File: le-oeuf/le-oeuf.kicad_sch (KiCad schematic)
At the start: 76 parts, among them J1 S2B-PH-K-S, SW1 PG1425, SW10 PG1425, SW11 PG1425, SW12 PG1425, SW13 PG1425, SW14 PG1425, SW15 PG1425, SW16 PG1425, SW17 PG1425, SW18 PG1425, SW19 PG1425, SW2 PG1425, SW20 PG1425, SW21 PG1425, SW22 PG1425, SW23 PG1425, SW24 PG1425, SW25 PG1425, SW26 PG1425, SW27 PG1425, SW28 PG1425, SW29 PG1425, SW3 PG1425, SW30 PG1425, SW31 PG1425, SW32 PG1425, SW33 PG1425, SW34 PG1425, SW35 PG1425, SW36 PG1425, SW37 PCM12SMTR, SW4 PG1425, SW5 PG1425, SW6 PG1425, SW7 PG1425, SW8 PG1425, SW9 PG1425, U1 Seeeduino Xiao nRF52840, U2 74HC595D,118

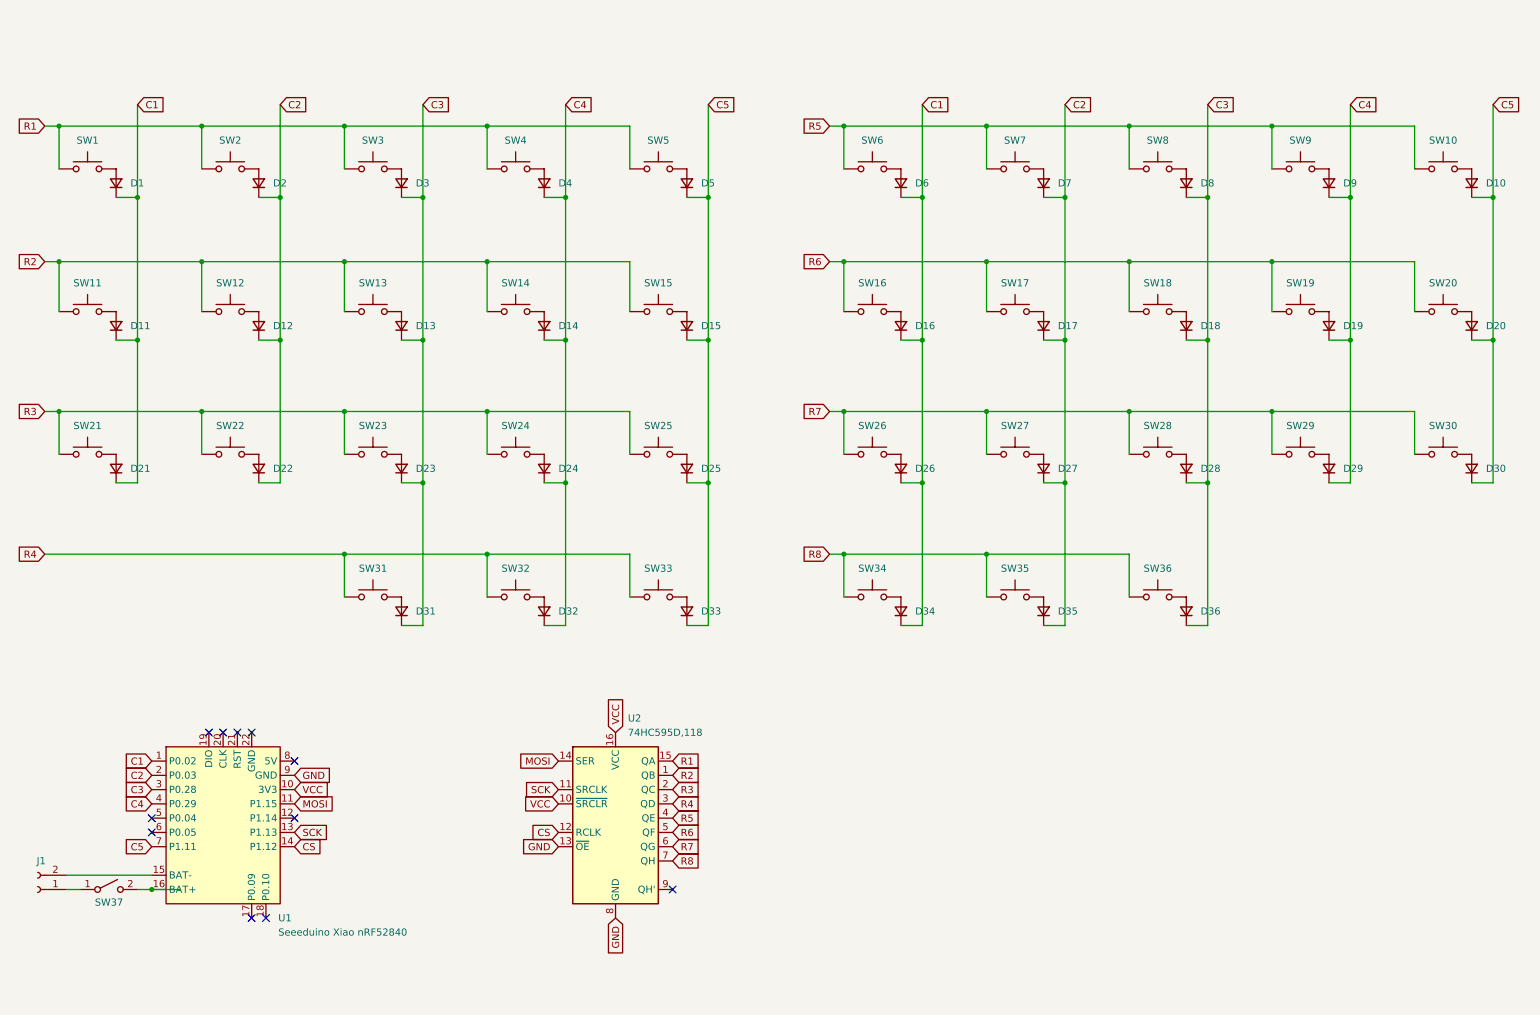
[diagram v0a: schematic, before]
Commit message: do not push this commit
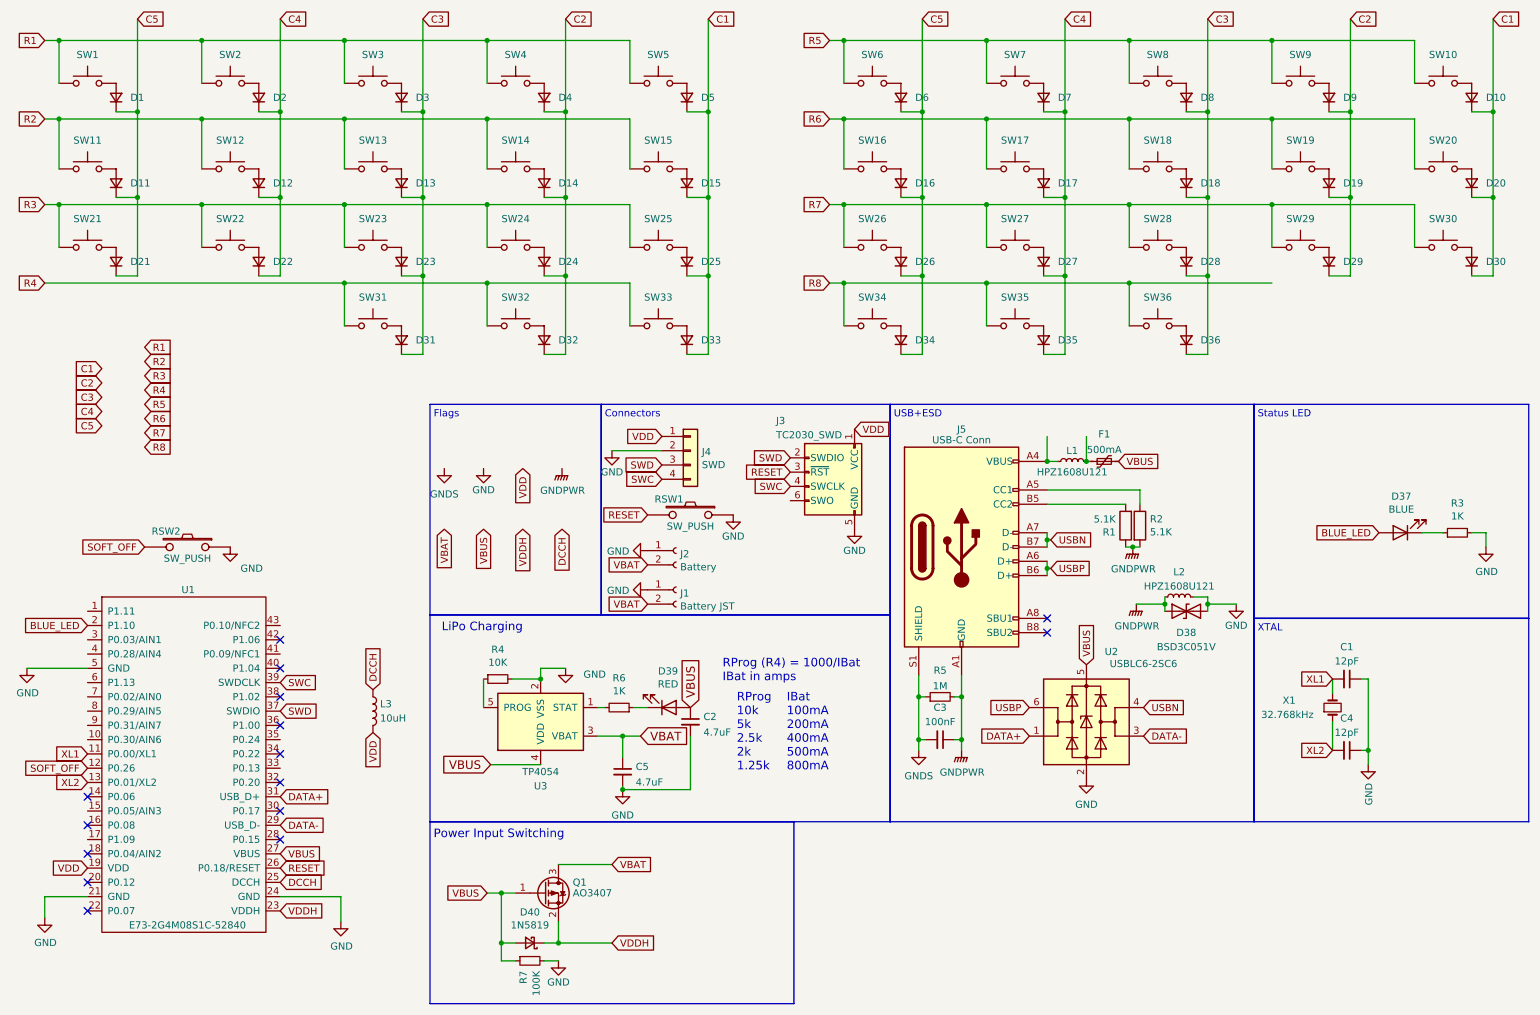
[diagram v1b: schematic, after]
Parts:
- removed J1: S2B-PH-K-S, Connector_JST:JST_PH_S2B-PH-K_1x02_P2.00mm_Horizontal, symbol Connector:Conn_01x02_Socket
- removed SW37: PCM12SMTR, Button_Switch_SMD:SW_SPDT_PCM12, symbol Switch:SW_SPST
- removed U1: Seeeduino Xiao nRF52840, le-oeuf:Xiao_nRF52840_AC_Reflow, symbol PCM_marbastlib-promicroish:Seeeduino_Xiao_nRF52840
- removed U2: 74HC595D,118, Package_SO:SOIC-16_3.9x9.9mm_P1.27mm, symbol 74xx:74HC595
- added C1, C4: 12pF, Capacitor_SMD:C_0603_1608Metric, symbol Device:C_Small
- added C2, C5: 4.7uF, Capacitor_SMD:C_0603_1608Metric, symbol Device:C_Small
- added C3: 100nF, Capacitor_SMD:C_0603_1608Metric, symbol Device:C_Small
- added D37: BLUE, LED_SMD:LED_1206_3216Metric, symbol Device:LED
- added D38: BSD3C051V, Diode_SMD:D_SOD-323, symbol Device:D_TVS
- added D39: RED, LED_SMD:LED_1206_3216Metric, symbol Device:LED
- added D40: 1N5819, Diode_SMD:D_SOD-323, symbol Device:D_Schottky_Small
- added F1: 500mA, Fuse:Fuse_1206_3216Metric, symbol Device:Polyfuse_Small
- added J1: Battery JST, Connector_JST:JST_ACH_BM02B-ACHSS-GAN-ETF_1x02-1MP_P1.20mm_Vertical, symbol Connector:Conn_01x02_Female
- added J2: Battery, Connector_PinHeader_2.00mm:PinHeader_1x02_P2.00mm_Vertical, symbol Connector:Conn_01x02_Female
- added J3: TC2030_SWD, PCM_marbastlib-various:CON_TC2030_outlined, symbol PCM_marbastlib-various:TC2030_SWD
- added J4: SWD, Connector_PinHeader_2.54mm:PinHeader_1x04_P2.54mm_Vertical, symbol Connector_Generic:Conn_01x04
- added J5: USB-C Conn, PCM_marbastlib-various:USB_C_Receptacle_HRO_TYPE-C-31-M-14, symbol Connector:USB_C_Receptacle_USB2.0
- added L1, L2: HPZ1608U121, Inductor_SMD:L_0603_1608Metric_Pad1.05x0.95mm_HandSolder, symbol Device:L_Small
- added L3: 10uH, Inductor_SMD:L_0603_1608Metric_Pad1.05x0.95mm_HandSolder, symbol Device:L
- added Q1: AO3407, Package_TO_SOT_SMD:SOT-23, symbol Device:Q_PMOS_GSD
- added R1, R2: 5.1K, Resistor_SMD:R_0603_1608Metric, symbol Device:R
- added R3, R6: 1K, Resistor_SMD:R_0603_1608Metric, symbol Device:R_Small
- added R4: 10K, Resistor_SMD:R_0603_1608Metric, symbol Device:R_Small
- added R5: 1M, Resistor_SMD:R_0603_1608Metric, symbol Device:R_Small
- added R7: 100K, Resistor_SMD:R_0603_1608Metric, symbol Device:R_Small
- added RSW1, RSW2: SW_PUSH, Button_Switch_SMD:Panasonic_EVQPUL_EVQPUC, symbol corne-cherry-rescue:SW_PUSH-kbd-corne-cherry-rescue
- added U1: E73-2G4M08S1C-52840, PCM_marbastlib-various:nRF52840_E73-2G4M08S1C, symbol nrfmicro:E73-2G4M08S1C-52840
- added U2: USBLC6-2SC6, Package_TO_SOT_SMD:TSOT-23-6, symbol Power_Protection:USBLC6-2SC6
- added U3: TP4054, Package_TO_SOT_SMD:SOT-23-5, symbol Battery_Management:MCP73831-3-OT
- added X1: 32.768kHz, Crystal:Crystal_SMD_MicroCrystal_CM9V-T1A-2Pin_1.6x1.0mm_HandSoldering, symbol Device:Crystal_Small
- SW1, SW10, SW11, SW12, SW13, SW14, SW15, SW16, SW17, SW18, SW19, SW2, SW20, SW21, SW22, SW23, SW24, SW25, SW26, SW27, SW28, SW29, SW3, SW30, SW31, SW32, SW33, SW34, SW35, SW36, SW4, SW5, SW6, SW7, SW8, SW9: footprint le-oeuf:Kailh-PG1425-X-Switch -> le-oeuf:CPG1316S01D02_mikeholscher
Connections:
- net C1: now also D10.1 (K), D15.1 (K), D20.1 (K), D25.1 (K), D30.1 (K), D33.1 (K), D5.1 (K); no longer D1.1 (K), D11.1 (K), D16.1 (K), D21.1 (K), D26.1 (K), D34.1 (K), D6.1 (K)
- net C2: now also D14.1 (K), D19.1 (K), D24.1 (K), D29.1 (K), D32.1 (K), D4.1 (K), D9.1 (K); no longer D12.1 (K), D17.1 (K), D2.1 (K), D22.1 (K), D27.1 (K), D35.1 (K), D7.1 (K)
- net C4: now also D12.1 (K), D17.1 (K), D2.1 (K), D22.1 (K), D27.1 (K), D35.1 (K), D7.1 (K); no longer D14.1 (K), D19.1 (K), D24.1 (K), D29.1 (K), D32.1 (K), D4.1 (K), D9.1 (K)
- net C5: now also D1.1 (K), D11.1 (K), D16.1 (K), D21.1 (K), D26.1 (K), D34.1 (K), D6.1 (K); no longer D10.1 (K), D15.1 (K), D20.1 (K), D25.1 (K), D30.1 (K), D33.1 (K), D5.1 (K)
- net GND: now also C1.1, C2.2, C4.1, C5.2, D38.2 (A2), J1.1 (Pin_1), J2.1 (Pin_1), J3.5 (GND), J4.2 (Pin_2), L2.2, R3.2, R4.2, R7.2, RSW1.1, RSW2.1, U1.21 (GND), U1.24 (GND), U1.5 (GND), U2.2 (GND), U3.2 (VSS)
- new net: D37.1 (K), R3.1
- new net: D39.1 (K), R6.1
- new net: J5.B5 (CC2), R1.2
- new net: F1.1, L1.2
- new net: R4.1, U3.5 (PROG)
- new net: J5.A4 (VBUS), J5.A9 (VBUS), J5.B4 (VBUS), J5.B9 (VBUS), L1.1
- new net: J5.A5 (CC1), R2.1
- new net: R6.2, U3.1 (STAT)
- new net BLUE_LED: D37.2 (A), U1.2 (P1.10)
- new net DATA+: U1.31 (USB_D+), U2.1 (I/O1)
- new net DATA-: U1.29 (USB_D-), U2.3 (I/O2)
- new net DCCH: L3.1, U1.25 (DCCH)
- new net GNDPWR: C3.1, D38.1 (A1), J5.A1 (GND), J5.A12 (GND), J5.B1 (GND), J5.B12 (GND), L2.1, R1.1, R2.2, R5.2
- new net GNDS: C3.2, J5.S1 (SHIELD), R5.1
- new net RESET: J3.3 (~{RST}), RSW1.2, U1.26 (P0.18/RESET)
- new net SOFT_OFF: RSW2.2, U1.12 (P0.26)
- new net SWC: J3.4 (SWCLK), J4.4 (Pin_4), U1.39 (SWDCLK)
- new net SWD: J3.2 (SWDIO), J4.3 (Pin_3), U1.37 (SWDIO)
- new net USBN: J5.A7 (D-), J5.B7 (D-), U2.4 (I/O2)
- new net USBP: J5.A6 (D+), J5.B6 (D+), U2.6 (I/O1)
- new net VBAT: C5.1, J1.2 (Pin_2), J2.2 (Pin_2), Q1.3 (D), U3.3 (VBAT)
- new net VBUS: C2.1, D39.2 (A), D40.2 (A), F1.2, Q1.1 (G), R7.1, U1.27 (VBUS), U2.5 (VBUS), U3.4 (VDD)
- new net VDD: J3.1 (VCC), J4.1 (Pin_1), L3.2, U1.19 (VDD)
- new net VDDH: D40.1 (K), Q1.2 (S), U1.23 (VDDH)
- new net XL1: C1.2, U1.11 (P0.00/XL1), X1.2
- new net XL2: C4.2, U1.13 (P0.01/XL2), X1.1
- no-connect marks 11 -> 15
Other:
- note added: "Connectors"
- note added: "Flags"
- note added: "IBat 100mA 200mA 400mA 500mA 800mA"
- note added: "LiPo Charging"
- note added: "Power Input Switching"
- note added: "RProg (R4) = 1000/IBat IBat in amps"
- note added: "RProg 10k 5k 2.5k 2k 1.25k"
- note added: "Status LED"
- note added: "USB+ESD"
- note added: "XTAL"
- moved on the sheet: D1, D10, D11, D12, D13, D14, D15, D16, D17, D18, D19, D2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

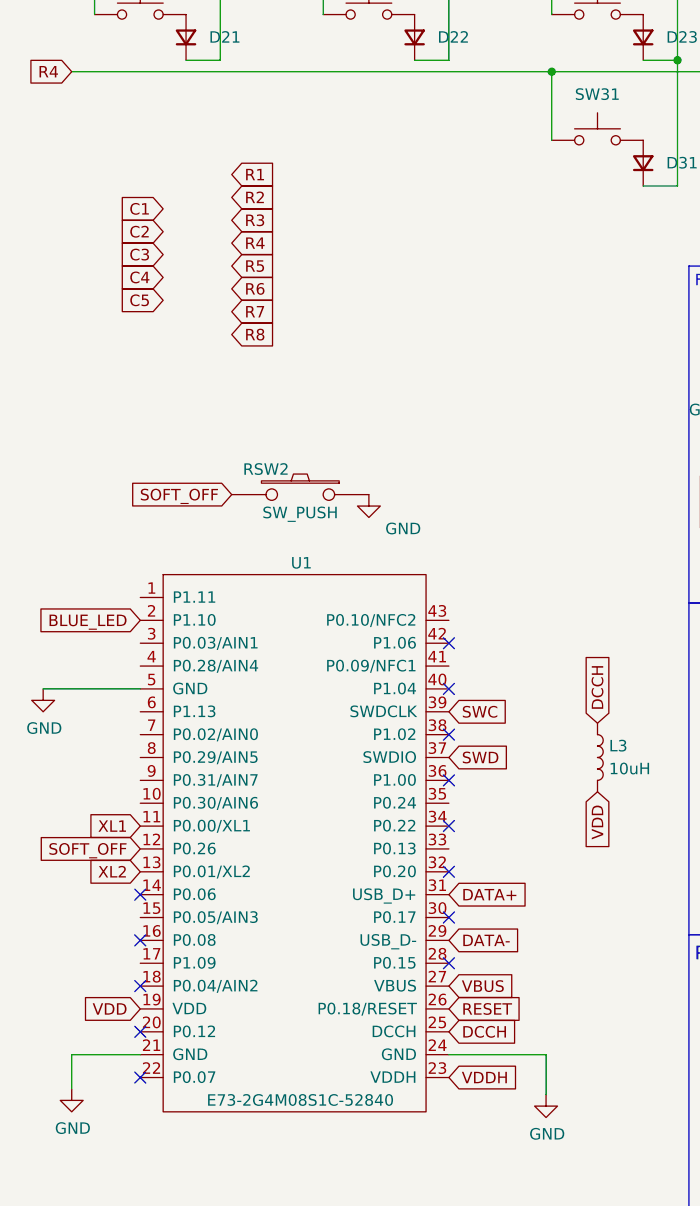
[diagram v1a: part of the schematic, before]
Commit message: finish routing
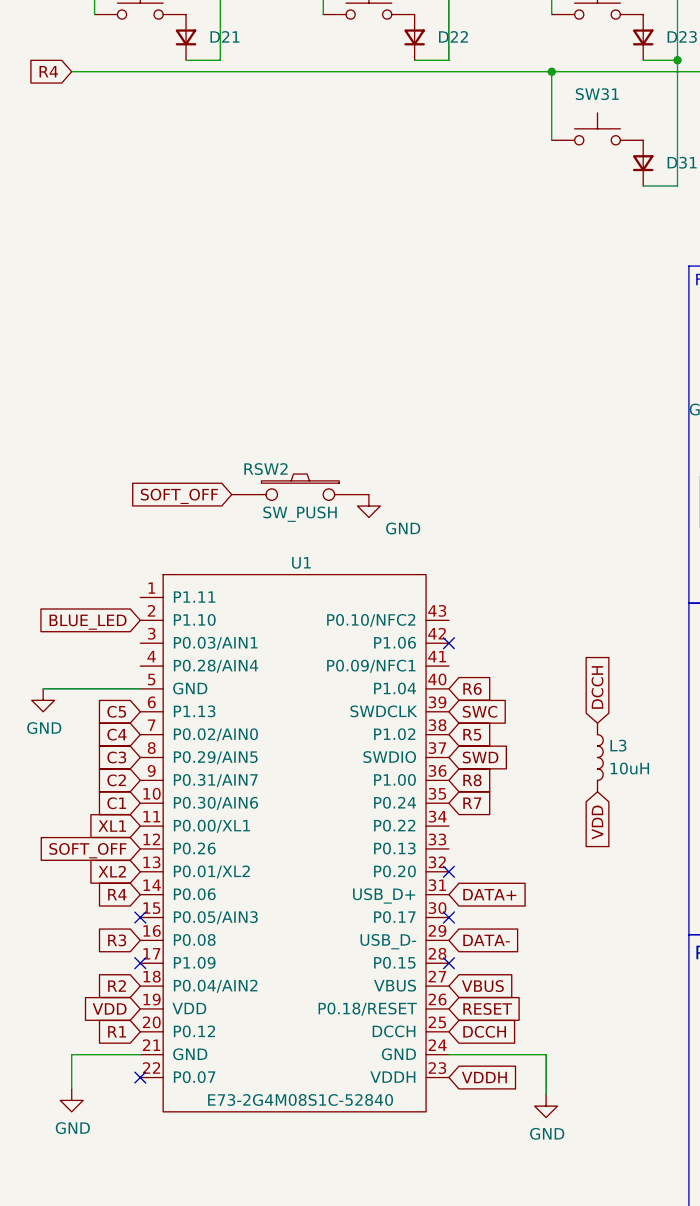
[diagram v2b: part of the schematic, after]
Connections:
- net C1: now also U1.10 (P0.30/AIN6)
- net C2: now also U1.9 (P0.31/AIN7)
- net C3: now also U1.8 (P0.29/AIN5)
- net C4: now also U1.7 (P0.02/AIN0)
- net C5: now also U1.6 (P1.13)
- net R1: now also U1.20 (P0.12)
- net R2: now also U1.18 (P0.04/AIN2)
- net R3: now also U1.16 (P0.08)
- net R4: now also U1.14 (P0.06)
- net R5: now also U1.38 (P1.02)
- net R6: now also U1.40 (P1.04)
- net R7: now also U1.35 (P0.24)
- net R8: now also U1.36 (P1.00)
- no-connect marks 15 -> 9

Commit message: import art
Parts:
- L1, L2, L3: footprint Inductor_SMD:L_0603_1608Metric_Pad1.05x0.95mm_HandSolder -> Inductor_SMD:L_0603_1608Metric
- X1: footprint Crystal:Crystal_SMD_MicroCrystal_CM9V-T1A-2Pin_1.6x1.0mm_HandSoldering -> Crystal:Crystal_SMD_MicroCrystal_CM9V-T1A-2Pin_1.6x1.0mm
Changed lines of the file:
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@@
 			)
 		)
-		(property "Footprint" "Crystal:Crystal_SMD_MicroCrystal_CM9V-T1A-2Pin_1.6x1.0mm_HandSoldering"
+		(property "Footprint" "Crystal:Crystal_SMD_MicroCrystal_CM9V-T1A-2Pin_1.6x1.0mm"
 			(at 249.555 141.605 0)
 			(effects
@@
 			)
 		)
-		(property "Footprint" "Inductor_SMD:L_0603_1608Metric_Pad1.05x0.95mm_HandSolder"
+		(property "Footprint" "Inductor_SMD:L_0603_1608Metric"
 			(at 78.74 142.24 0)
 			(effects
@@
 			)
 		)
-		(property "Footprint" "Inductor_SMD:L_0603_1608Metric_Pad1.05x0.95mm_HandSolder"
+		(property "Footprint" "Inductor_SMD:L_0603_1608Metric"
 			(at 203.2 97.79 0)
 			(effects
@@
 			)
 		)
-		(property "Footprint" "Inductor_SMD:L_0603_1608Metric_Pad1.05x0.95mm_HandSolder"
+		(property "Footprint" "Inductor_SMD:L_0603_1608Metric"
 			(at 222.25 121.92 0)
 			(effects
